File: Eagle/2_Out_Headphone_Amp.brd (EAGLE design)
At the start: 100 x 80 mm, 29 parts, among them IC1 OPA2134P, IC2 OPA2134P, IC3 OPA2134P

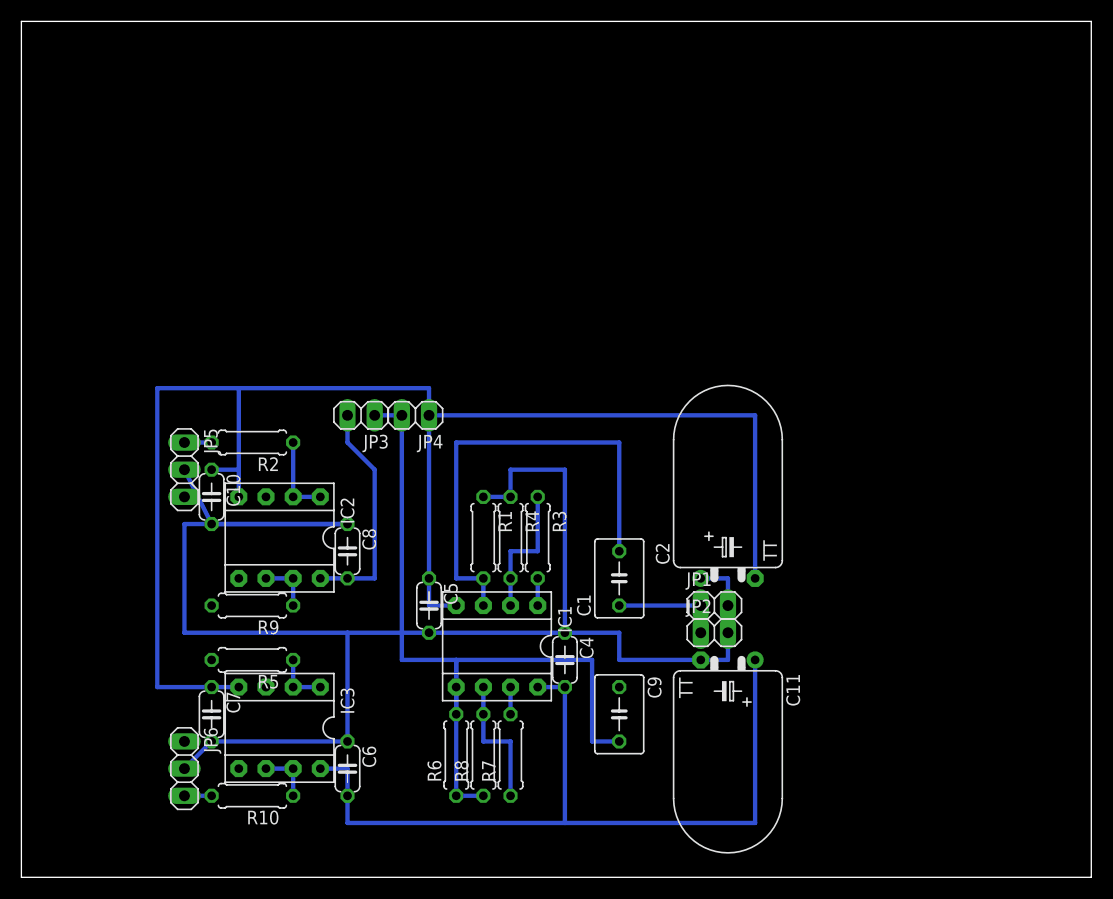
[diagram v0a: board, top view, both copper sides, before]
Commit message: 基板設計図微調整前
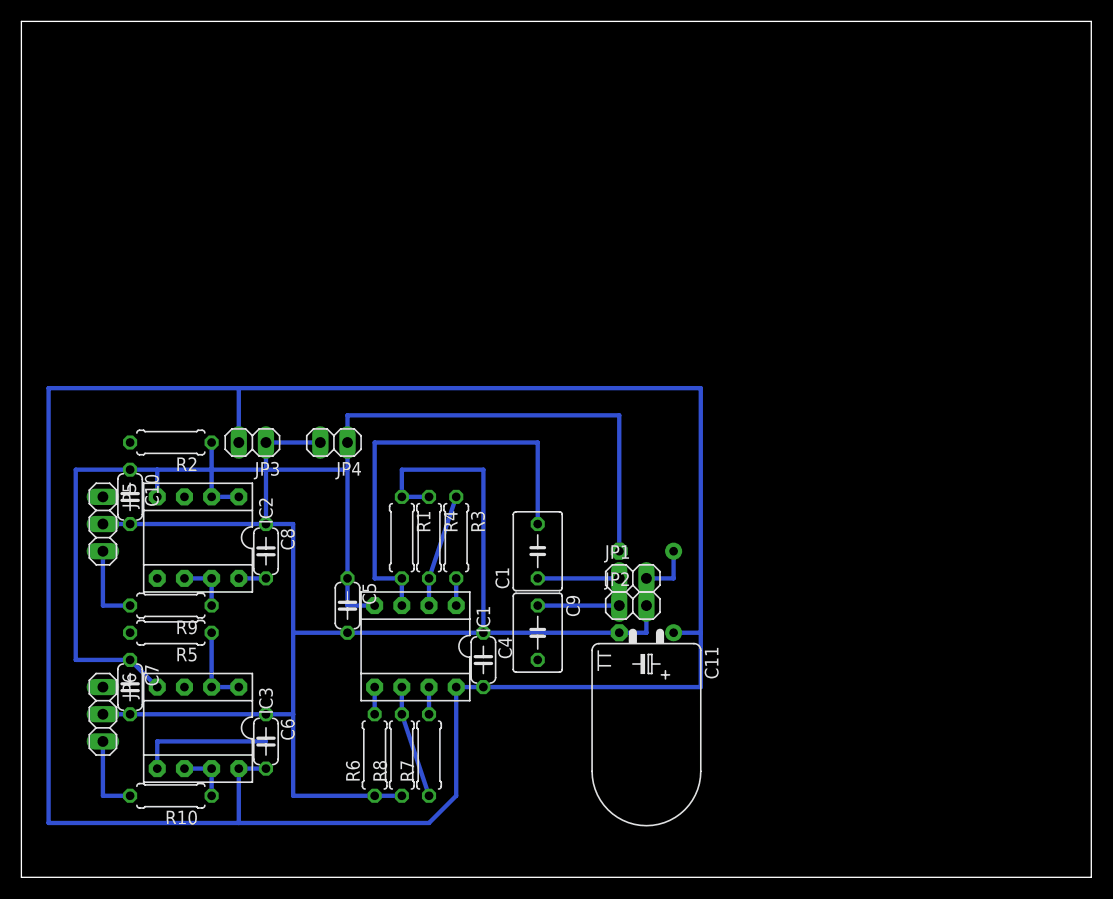
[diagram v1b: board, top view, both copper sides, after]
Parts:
- moved C9 10.8 mm to (48.3, 22.9)
- moved JP3 10.5 mm to (21.6, 40.6)
- moved JP5 9.16 mm to (7.62, 33.0)
- moved JP6 9.16 mm to (7.62, 15.2)
- moved C1 8.03 mm to (48.3, 30.5)
- moved C11 8.03 mm to (58.4, 22.9)
- moved C2 8.03 mm to (58.4, 30.5), flipped to the bottom
- moved C7 8.03 mm to (10.2, 17.8)
- moved C6 8.03 mm to (22.9, 12.7)
- moved R5 8.03 mm to (14.0, 22.9)
- moved JP1 8.03 mm to (57.1, 27.9)
- moved JP2 8.03 mm to (57.1, 25.4)
- moved JP4 8.03 mm to (29.2, 40.6)
- moved IC1 7.62 mm to (36.8, 21.6)
- moved C10 7.62 mm to (10.2, 35.6)
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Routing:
- net V+: track 97.6 -> 219.5 mm
- net GND: track 204.9 -> 154.9 mm
- net V-: track 142.2 -> 112.8 mm
- net N$10: track 27.9 -> 2.54 mm
- net N$12: track 2.54 -> 15.2 mm
- net N$9: track 0.00 -> 7.62 mm
- net N$15: track 0.00 -> 7.62 mm
- net N$16: track 2.54 -> 7.62 mm
- net N$2: track 43.2 -> 40.6 mm
- net N$6: track 2.54 -> 0.00 mm
- net N$7: track 5.08 -> 7.62 mm
- net N$3: track 12.7 -> 10.6 mm
- net N$11: track 12.7 -> 10.6 mm

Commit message: 基板設計図 抵抗を立てる前
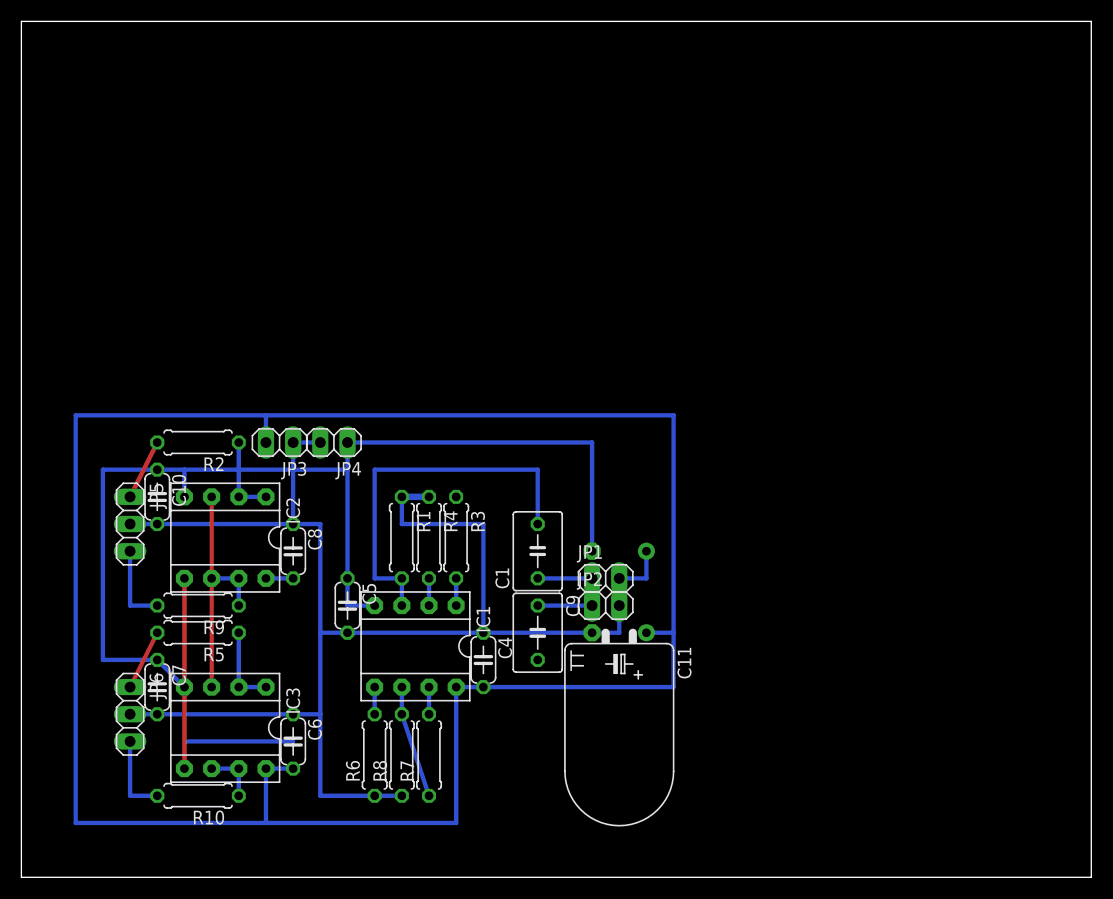
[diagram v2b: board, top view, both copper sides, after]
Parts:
- moved R10 2.54 mm to (16.5, 7.62)
- moved R2 2.54 mm to (16.5, 40.6)
- moved R5 2.54 mm to (16.5, 22.9)
- moved R9 2.54 mm to (16.5, 25.4)
- moved JP5 2.54 mm to (10.2, 33.0)
- moved JP6 2.54 mm to (10.2, 15.2)
- moved C10 2.54 mm to (12.7, 35.6)
- moved C11 2.54 mm to (55.9, 22.9)
- moved C2 2.54 mm to (55.9, 30.5)
- moved C6 2.54 mm to (25.4, 12.7)
- moved C7 2.54 mm to (12.7, 17.8)
- moved C8 2.54 mm to (25.4, 30.5)
- moved IC2 2.54 mm to (19.1, 31.8)
- moved IC3 2.54 mm to (19.1, 14.0)
- moved JP1 2.54 mm to (54.6, 27.9)
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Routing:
- net N$4: track 2.54 -> 20.3 mm
- net N$12: track 15.2 -> 33.0 mm
- net V+: track 219.5 -> 203.2 mm
- net GND: track 154.9 -> 139.7 mm
- net V-: track 112.8 -> 102.7 mm
- net N$3: track 10.6 -> 2.54 mm
- net N$8: track 0.00 -> 5.68 mm
- net N$6: track 0.00 -> 5.68 mm
- net N$2: track 40.6 -> 35.6 mm
- net N$9: track 7.62 -> 5.08 mm
- net N$1: track 7.62 -> 5.08 mm
